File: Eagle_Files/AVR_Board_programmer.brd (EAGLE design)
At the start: 39.6 x 46.5 mm, 22 parts, among them J1 10118192-0001LF, U1 CP2102N-A01-GQFN20

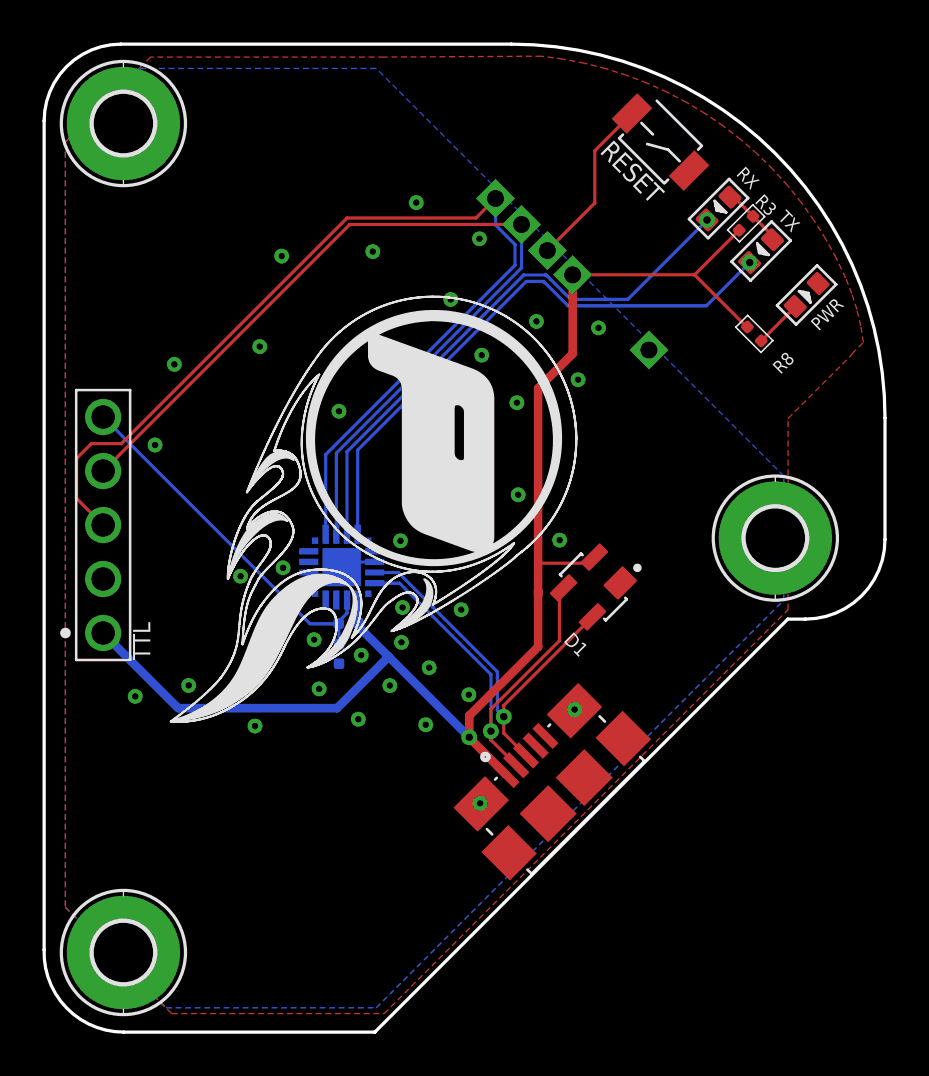
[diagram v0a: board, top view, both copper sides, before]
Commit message: Renamed boards, Fixed programmer
 - Renamed boards to more closely match change in spec/design revision
 - Added required components to usb serial board stack
   - Fixes https://github.com/pyr0ball/pyr0piezo/issues/9
 - Minor change to voltage values to stay consistent with local tests
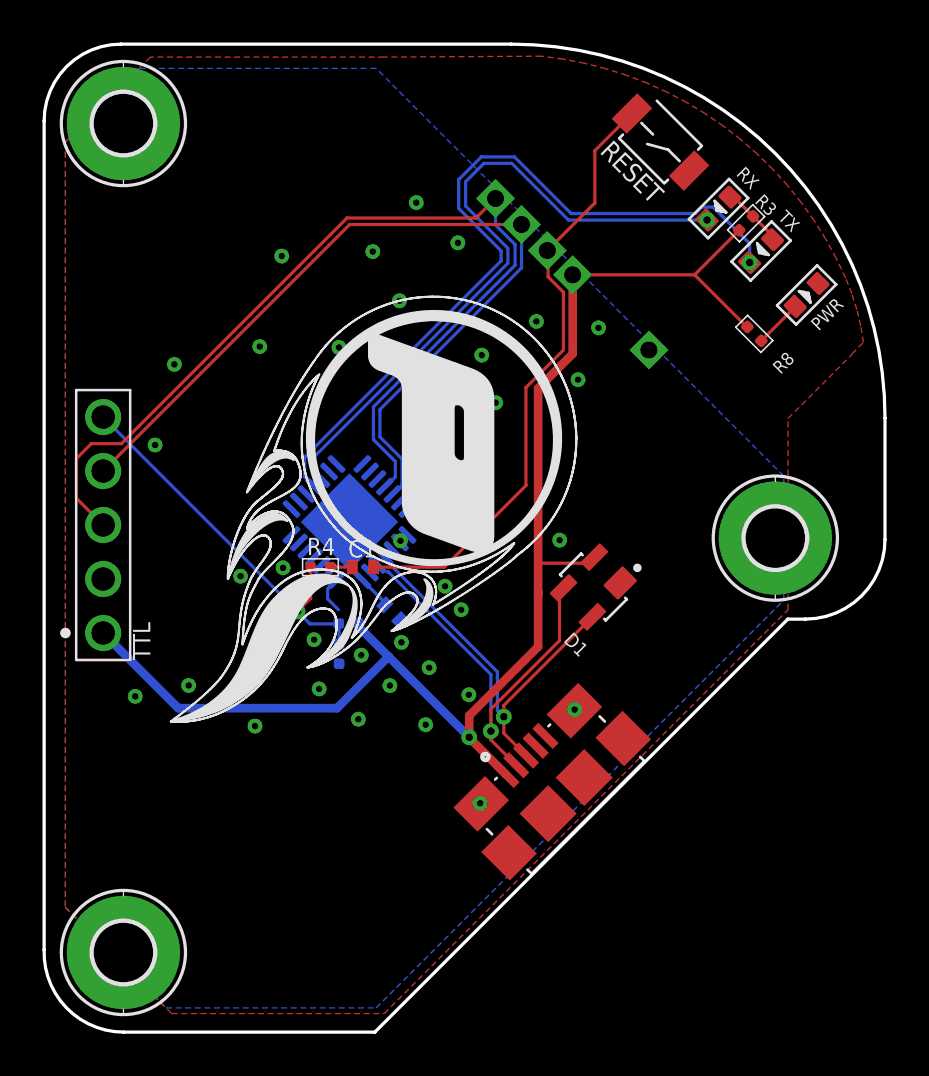
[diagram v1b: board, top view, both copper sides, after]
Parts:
- added C1, C2: 0.1uF, PiezoFFC:CAPC1005X50
- added R4: 10K, PiezoFFC:R0402
- U1: value CP2102N-A01-GQFN20 -> CP2102N-A01-GQFN28; device PiezoFFC:SILABS_QFN20 -> PiezoFFC:QFN50P500X500X80-29N
- moved U$2 10.1 mm to (14.4, 24.0), turned to 180 degrees
- moved U1 2.16 mm to (14.4, 24.1), turned to 45 degrees
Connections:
- new net PGM_RST: C1.2, R4.2, U1.28
- net 5V_DC: now also C2.2
- net GND: now also C2.1, U1.29; no longer U1.12, U1.21
- net RST: now also C1.1
- net RXD: now also U1.26; no longer U1.18
- net TXD: now also U1.25; no longer U1.17
- net TXT: now also U1.18; no longer U1.20
- net VBUS: now also R4.1
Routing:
- net RST: track 8.10 -> 29.0 mm
- net TXT: track 27.0 -> 36.2 mm
- net RXT: track 26.3 -> 31.6 mm
- net GND: track 3.51 -> 0.00 mm
- net VBUS: track 17.4 -> 20.3 mm, vias 0 -> 1
- net TXD: track 48.3 -> 45.8 mm
- net RXD: track 42.7 -> 40.6 mm
- net PGM_RST: track 0.00 -> 1.04 mm
- net 5V_DC: track 67.7 -> 68.3 mm
